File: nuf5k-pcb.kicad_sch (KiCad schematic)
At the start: 209 parts, among them J1 AVR-ISP-6, J2 1734366-1, J3 1734366-1, J4 1734366-1, SW0 KEYSW, SW1 KEYSW, SW10 KEYSW, SW11 KEYSW, SW12 KEYSW, SW13 KEYSW, SW14 KEYSW, SW15 KEYSW, SW16 KEYSW, SW17 KEYSW, SW18 KEYSW, SW19 KEYSW, SW2 KEYSW, SW20 KEYSW, SW21 KEYSW, SW22 KEYSW, SW23 KEYSW, SW24 KEYSW, SW25 KEYSW, SW26 KEYSW, SW27 KEYSW, SW28 KEYSW, SW29 KEYSW, SW3 KEYSW, SW30 KEYSW, SW31 KEYSW, SW32 KEYSW, SW33 KEYSW, SW34 KEYSW, SW35 KEYSW, SW36 KEYSW, SW37 KEYSW, SW38 KEYSW, SW39 KEYSW, SW4 KEYSW, SW40 KEYSW, SW41 KEYSW, SW42 KEYSW, SW43 KEYSW, SW44 KEYSW, SW45 KEYSW, SW46 KEYSW, SW47 KEYSW, SW48 KEYSW, SW49 KEYSW, SW5 KEYSW, SW50 KEYSW, SW51 KEYSW, SW52 KEYSW, SW53 KEYSW, SW54 KEYSW, SW55 KEYSW, SW56 KEYSW, SW57 KEYSW, SW58 KEYSW, SW59 KEYSW, SW6 KEYSW, SW60 KEYSW, SW61 KEYSW, SW62 KEYSW, SW63 KEYSW, SW64 KEYSW, SW65 KEYSW, SW66 KEYSW, SW67 KEYSW, SW68 KEYSW, SW69 KEYSW, SW7 KEYSW, SW70 KEYSW, SW71 KEYSW, SW72 KEYSW, SW73 KEYSW, SW74 KEYSW, SW75 KEYSW, SW76 KEYSW, SW77 KEYSW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

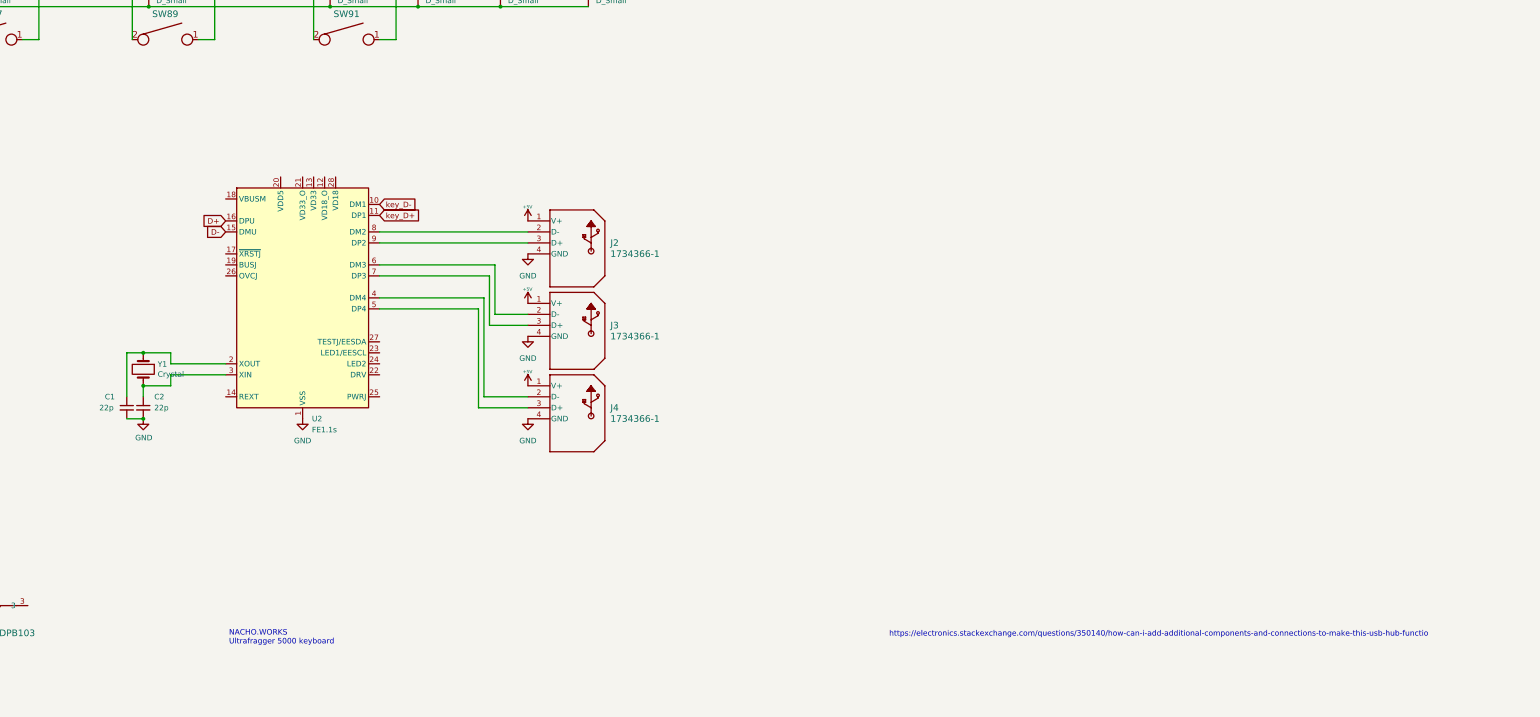
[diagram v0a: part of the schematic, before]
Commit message: FE1.1s works
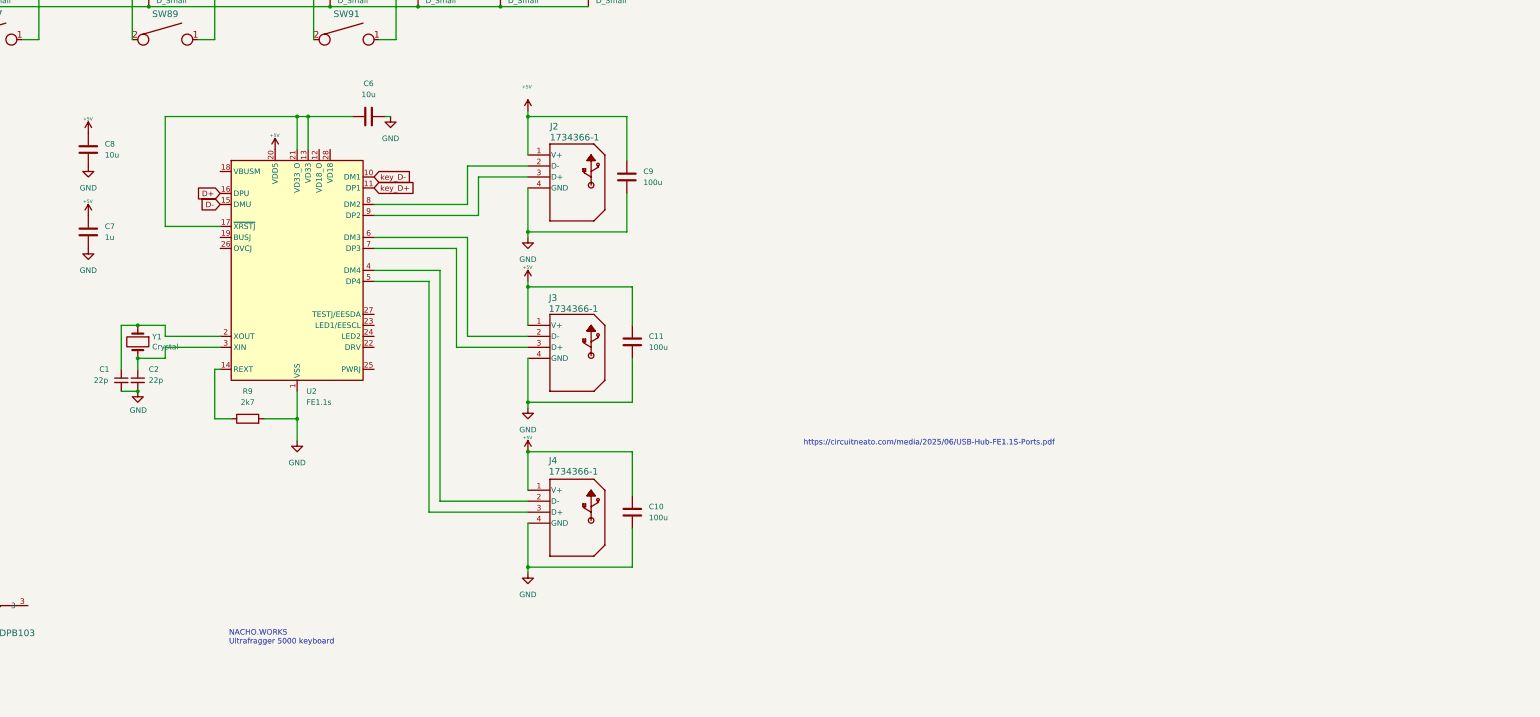
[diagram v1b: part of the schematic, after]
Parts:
- added C10, C11, C9: 100u, Capacitor_SMD:C_0201_0603Metric, symbol Device:C
- added C6, C8: 10u, Capacitor_SMD:C_0201_0603Metric, symbol Device:C
- added C7: 1u, Capacitor_SMD:C_0201_0603Metric, symbol Device:C
- added R9: 2k7, symbol Device:R
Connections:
- net +5V: now also U2.20 (VDD5), C10.2, C11.2, C7.2, C8.2, C9.2
- net GND: now also C10.1, C11.1, C6.2, C7.1, C8.1, C9.1, R9.2
- net at U2.13 (VD33): now also U2.17 (~{XRSTJ}), U2.21 (VD33_O), C6.1
- net at U2.14 (REXT): now also R9.1
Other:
- note added: "https://circuitneato.com/media/2025/06/USB-Hub-FE1.1S-Ports.pdf"
- note removed: "https://electronics.stackexchange.com/questions/350140/how-can-i-add-additional-components-and-connections-to-make-this-usb-hub-functio"
- moved on the sheet: C1, C2, J2, J3, J4, U2, Y1
